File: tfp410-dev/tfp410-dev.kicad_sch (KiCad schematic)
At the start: 2 parts, among them U1 TFP410PAP

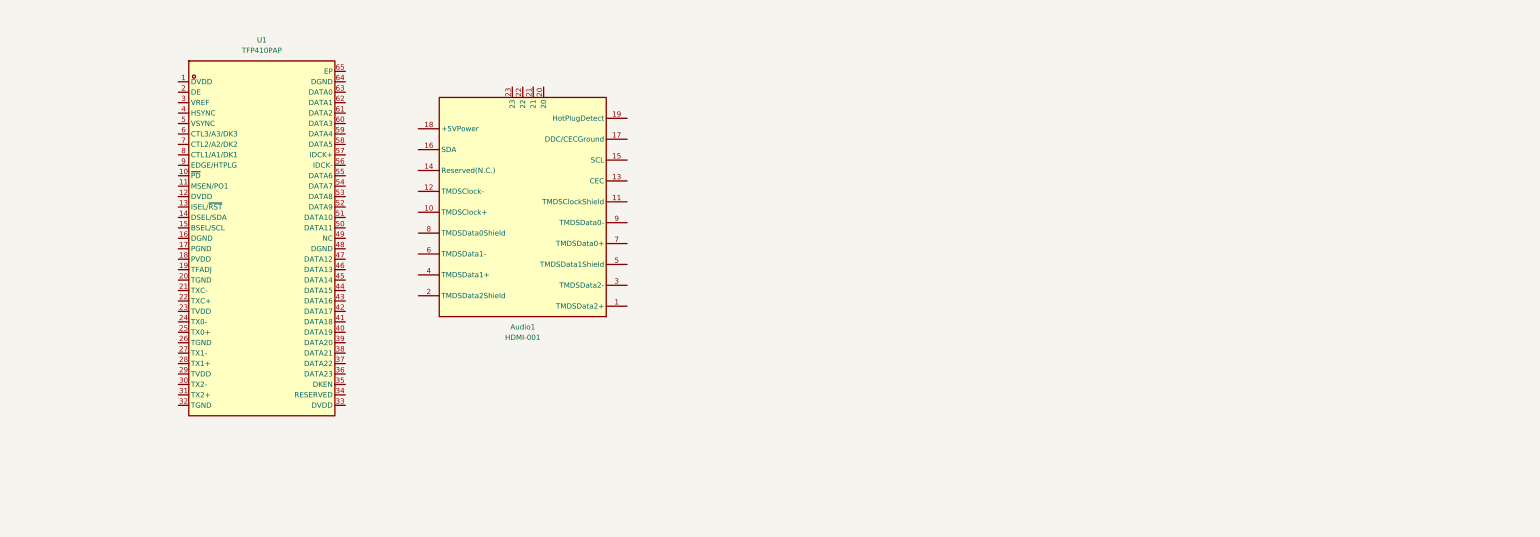
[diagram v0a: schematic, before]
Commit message: making schematics...
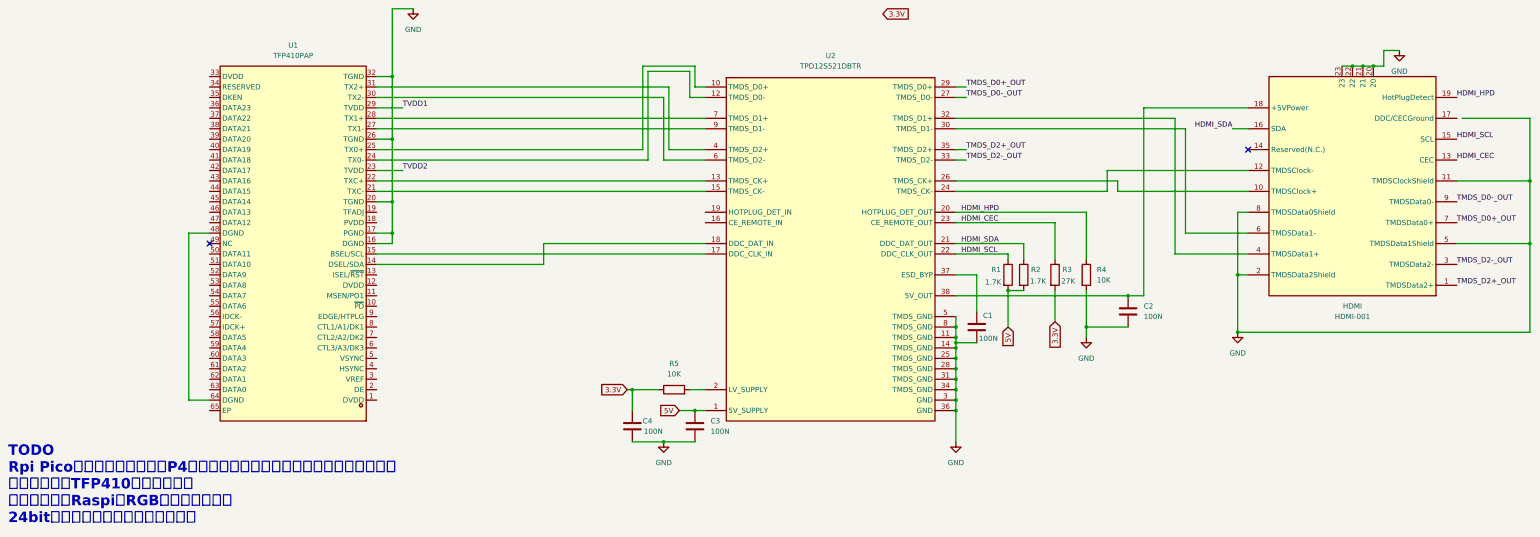
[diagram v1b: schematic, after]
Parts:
- added C1, C2, C3, C4: 100N, symbol Device:C
- added R1, R2: 1.7K, symbol Device:R
- added R3: 27K, symbol Device:R
- added R4, R5: 10K, symbol Device:R
- added U2: TPD12S521DBTR, easyeda2kicad:TSSOP-38_L9.7-W4.4-P0.50-LS6.4-BL, symbol easyeda2kicad:TPD12S521DBTR
- renumbered Audio1 to HDMI
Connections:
- net at U1.14 (DSEL/SDA): now also U2.18 (DDC_DAT_IN)
- net at U1.15 (BSEL/SCL): now also U2.17 (DDC_CLK_IN)
- net GND: now reaches U1.16 (DGND)
- net GND: now also HDMI.11 (TMDSClockShield), HDMI.2 (TMDSData2Shield), HDMI.20, HDMI.21, HDMI.22, HDMI.23, HDMI.5 (TMDSData1Shield), HDMI.8 (TMDSData0Shield), U1.17 (PGND), U1.20 (TGND), U1.26 (TGND), U1.32 (TGND), C1.2, C2.2, C3.2, C4.2, R4.2, U2.11 (TMDS_GND), U2.14 (TMDS_GND), U2.25 (TMDS_GND), U2.28 (TMDS_GND), U2.3 (GND), U2.31 (TMDS_GND), U2.34 (TMDS_GND), U2.36 (GND), U2.5 (TMDS_GND), U2.8 (TMDS_GND)
- net at U1.21 (TXC-): now also U2.15 (TMDS_CK-)
- net at U1.22 (TXC+): now also U2.13 (TMDS_CK+)
- net TVDD2: now reaches U1.23 (TVDD)
- net at U1.24 (TX0-): now also U2.12 (TMDS_D0-)
- net at U1.25 (TX0+): now also U2.10 (TMDS_D0+)
- net at U1.27 (TX1-): now also U2.9 (TMDS_D1-)
- net at U1.28 (TX1+): now also U2.7 (TMDS_D1+)
- net TVDD1: now reaches U1.29 (TVDD)
- net at U1.30 (TX2-): now also U2.6 (TMDS_D2-)
- net at U1.31 (TX2+): now also U2.4 (TMDS_D2+)
- net at U1.48 (DGND): now also U1.64 (DGND)
- net TMDS_D2+_OUT: now reaches HDMI.1 (TMDSData2+)
- net TMDS_D2+_OUT: now also U2.35 (TMDS_D2+)
- net at HDMI.10 (TMDSClock+): now also U2.26 (TMDS_CK+)
- net at HDMI.12 (TMDSClock-): now also U2.24 (TMDS_CK-)
- net HDMI_CEC: now reaches HDMI.13 (CEC)
- net HDMI_CEC: now also R3.1, U2.23 (CE_REMOTE_OUT)
- net HDMI_SCL: now reaches HDMI.15 (SCL)
- net HDMI_SCL: now also R1.1, U2.22 (DDC_CLK_OUT)
- net HDMI_SDA: now reaches HDMI.16 (SDA)
- net HDMI_SDA: now also R2.1, U2.21 (DDC_DAT_OUT)
- net at HDMI.18 (+5VPower): now also C2.1, U2.38 (5V_OUT)
- net HDMI_HPD: now reaches HDMI.19 (HotPlugDetect)
- net HDMI_HPD: now also R4.1, U2.20 (HOTPLUG_DET_OUT)
- net TMDS_D2-_OUT: now reaches HDMI.3 (TMDSData2-)
- net TMDS_D2-_OUT: now also U2.33 (TMDS_D2-)
- net at HDMI.4 (TMDSData1+): now also U2.32 (TMDS_D1+)
- net at HDMI.6 (TMDSData1-): now also U2.30 (TMDS_D1-)
- net TMDS_D0+_OUT: now reaches HDMI.7 (TMDSData0+)
- net TMDS_D0+_OUT: now also U2.29 (TMDS_D0+)
- net TMDS_D0-_OUT: now reaches HDMI.9 (TMDSData0-)
- net TMDS_D0-_OUT: now also U2.27 (TMDS_D0-)
- new net: R5.2, U2.2 (LV_SUPPLY)
- new net: C1.1, U2.37 (ESD_BYP)
- new net 3.3V: C4.1, R3.2, R5.1
- new net 5V: C3.1, R1.2, R2.2, U2.1 (5V_SUPPLY)
- no-connect marks 0 -> 2
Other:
- note added: "TODO Rpi Pico互換のピンヘッダでP4評価基板を刺すためのシンボルを作成する。 そのうえで、TFP410へ接続する。 動作確認にはRaspiのRGB出力が使える。 24bit入力に対応するべきかどうか？"
- moved on the sheet: HDMI, U1
